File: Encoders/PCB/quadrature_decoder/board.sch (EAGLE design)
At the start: 14 parts, among them IC1 LFLS7366R, IC2 LFLS7366R, IC3 LFLS7366R, IC4 LFLS7366R, IC5 LFLS7366R, IC6 LFLS7366R

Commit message: changed pcb libs.
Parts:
- removed U$7: DUE(NORMAL), DUElib130425:DUE(NORMAL)
- added U$1: DUE(ENCODER), DUElib130425:DUE(ENCODER)
- CON1, CON2, CON3: device con-lstb:MA05-1 -> encoder_project:MA05-1
- CON4, CON5, CON6: device con-lstb:MA05-1 -> encoder_project:MA05-1(BOTTOM)
- UART: device con-lstb:MA03-1 -> encoder_project:MA03-1
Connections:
- net 3.3V: now also U$1.3V3; no longer U$7.3V3
- net 5V: now also U$1.5V; no longer U$7.5V
- net FCKI: now also U$1.DAC1; no longer U$7.DAC1
- net GND: now also U$1.5V_ICSP; no longer U$7.5V_ICSP
- net MISO: now also U$1.MISO_ICSP; no longer U$7.MISO_ICSP
- net MOSI: now also U$1.MOSI_ICSP; no longer U$7.MOSI_ICSP
- net N$3: now also U$1.TX1; no longer U$7.TX1
- net N$4: now also U$1.RX1; no longer U$7.RX1
- net SCK: now also U$1.SCK_ICSP; no longer U$7.SCK_ICSP
- net SS1: now also U$1.4; no longer U$7.4
- net SS2: now also U$1.5; no longer U$7.5
- net SS3: now also U$1.6; no longer U$7.6
- net SS4: now also U$1.7; no longer U$7.7
- net SS5: now also U$1.8; no longer U$7.8
- net SS6: now also U$1.9; no longer U$7.9

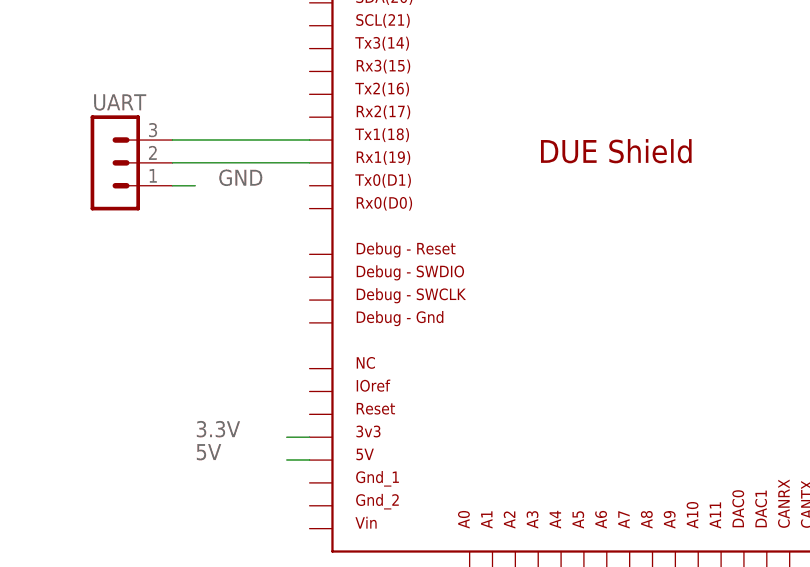
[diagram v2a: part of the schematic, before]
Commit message: rerouted
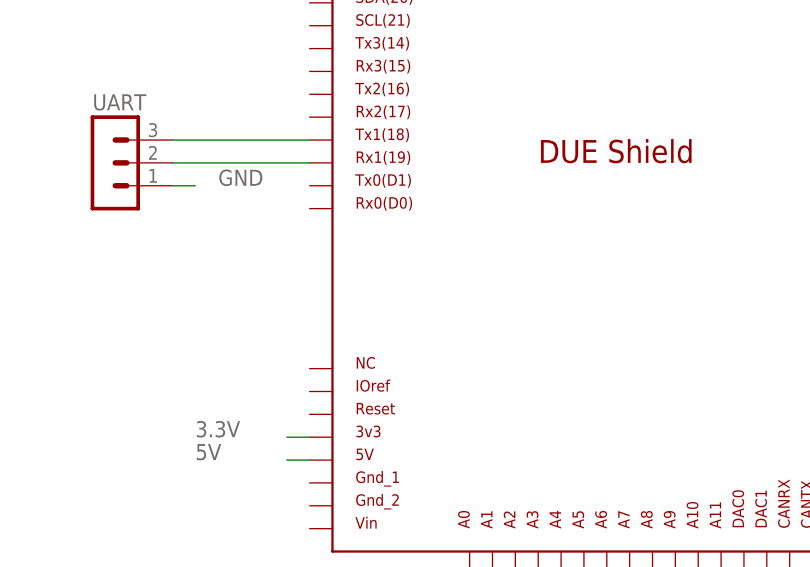
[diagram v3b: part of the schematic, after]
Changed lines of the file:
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@@
 <?xml version="1.0" encoding="utf-8"?>
 <!DOCTYPE eagle SYSTEM "eagle.dtd">
-<eagle version="8.3.1">
+<eagle version="8.2.0">
 <drawing>
 <settings>
 <setting alwaysvectorfont="no"/>
-<setting keepoldvectorfont="yes"/>
 <setting verticaltext="up"/>
 </settings>
